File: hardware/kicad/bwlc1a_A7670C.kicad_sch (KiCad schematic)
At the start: 54 parts, among them J3 Nano SIM, J5 BWIPX-1-001E, Q1 S8050, Q2 S8050, Q5 S8050, Q6 S8050, U2 A7670C_24x24mm, U5 MIC29302WU

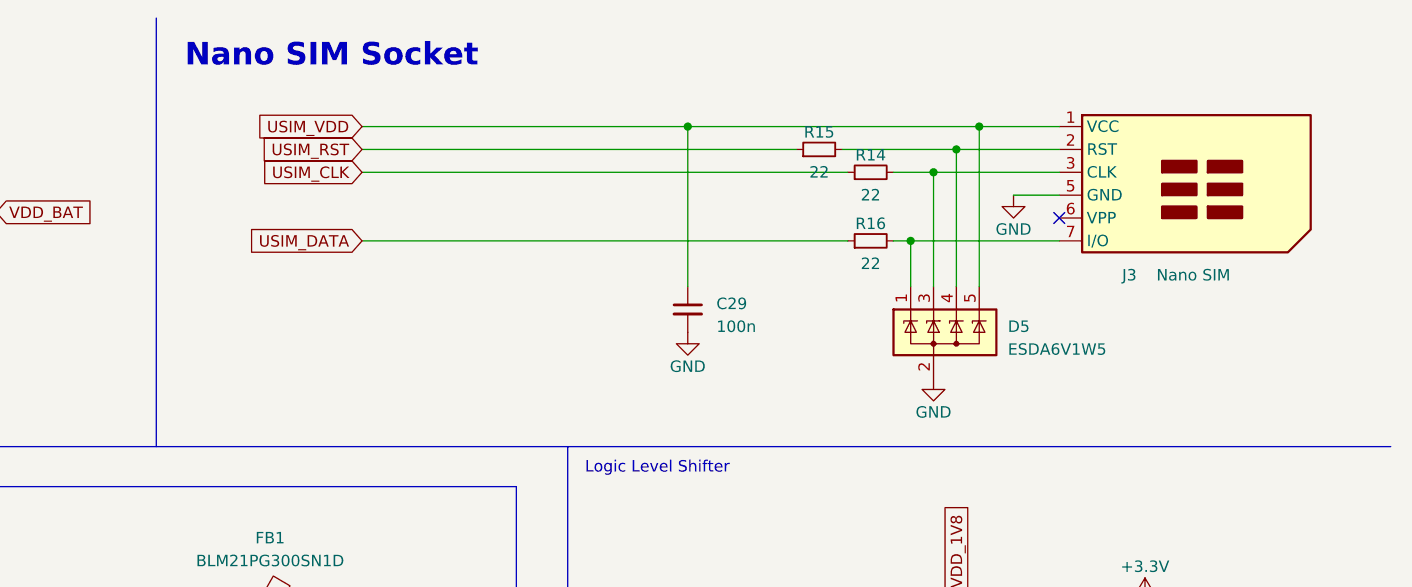
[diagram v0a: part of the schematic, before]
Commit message: Update PCB
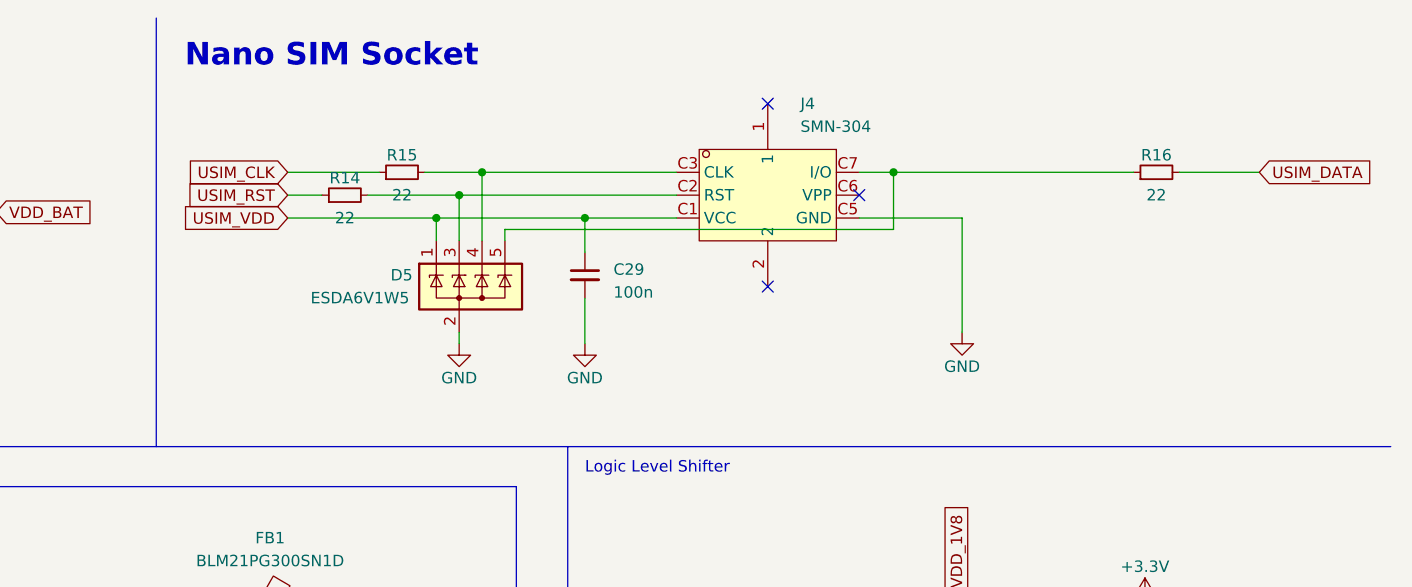
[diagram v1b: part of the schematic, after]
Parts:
- removed J3: Nano SIM, GCT_SIM8051-6-0-14-00-X-REVD:GCT_SIM8051-6-0-14-00-X-REVD, symbol Connector:SIM_Card
- added J4: SMN-304, SIM-SMD_SMN-304:SIM-SMD_SMN-304, symbol SIM-SMD_SMN-304:SMN-304
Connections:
- net GND: now also J4.C5 (GND)
- net USIM_CLK: now also R15.1; no longer R14.1
- net USIM_DATA: now also R16.2; no longer R16.1
- net USIM_RST: now also R14.1; no longer R15.1
- net USIM_VDD: now also D5.1 (K), J4.C1 (VCC); no longer D5.5 (K)
- net at D5.3 (K), R14.2: now also J4.C2 (RST)
- net at D5.4 (K), R15.2: now also J4.C3 (CLK)
- new net: D5.5 (K), J4.C7 (I/O), R16.1
- no-connect marks 36 -> 38
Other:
- moved on the sheet: C29, D5, R14, R15, R16
